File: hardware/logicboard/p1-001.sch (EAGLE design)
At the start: 25 parts, among them IC1 74LS07N, U1 TLC5940-NT, X1 HIROSE-DX10LM1-14SE

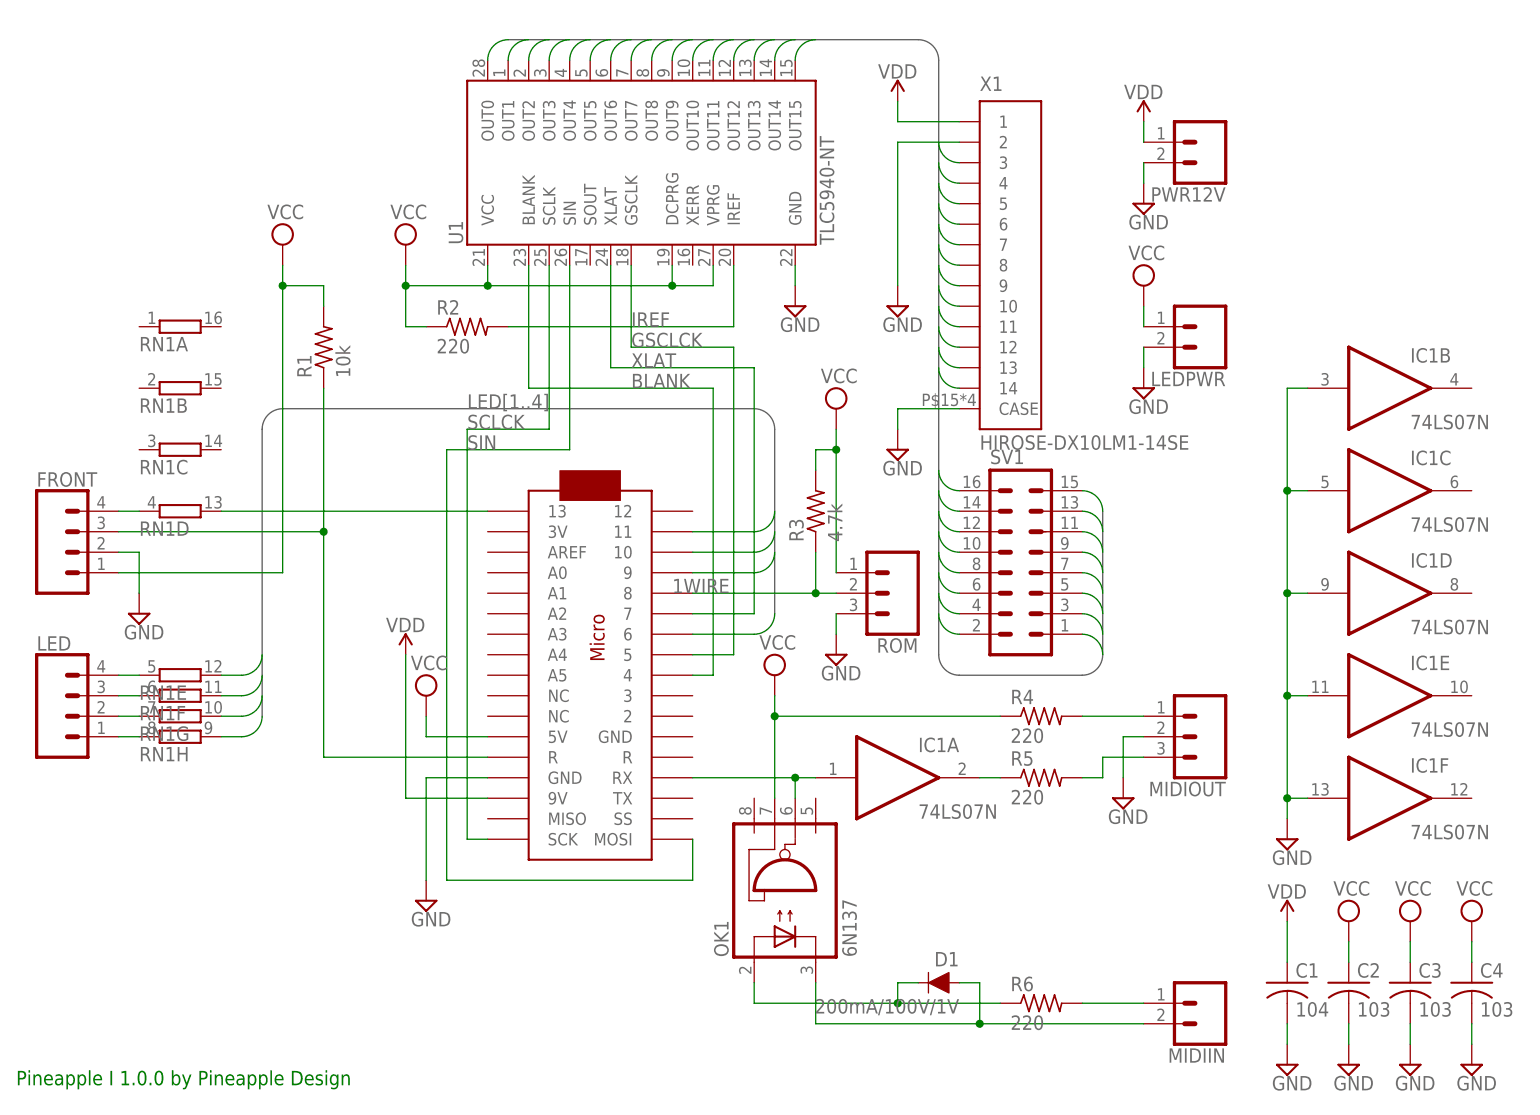
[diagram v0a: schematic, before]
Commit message: Relay.
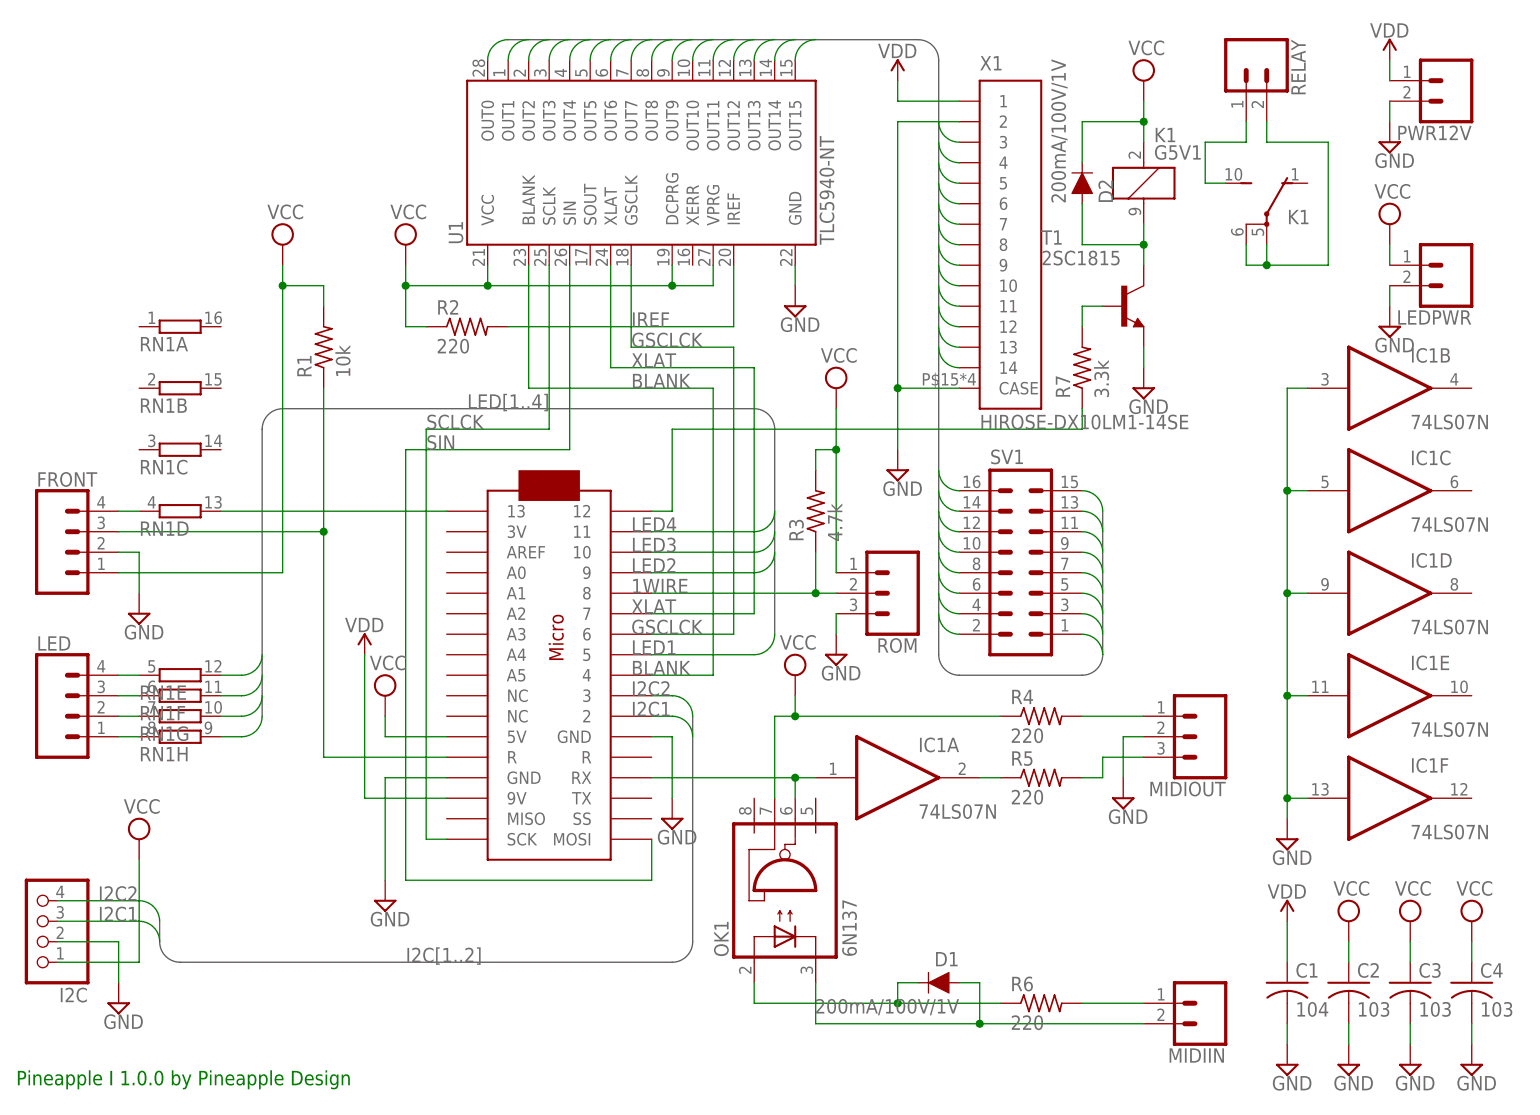
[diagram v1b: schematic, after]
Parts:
- added D2: 200mA/100V/1V, SparkFun-DiscreteSemi:DIODE-1N4148
- added I2C: (no value), pinhead:PINHD-1X4
- added K1: G5V1, relay:G5V1
- added R7: 3.3k, resistor:R-US_0204/5
- added RELAY: (no value), SparkFun-Connectors:CONN_02JST-PTH-2
- added T1: 2SC1815, transistor:2SC1815
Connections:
- new net I2C1: I2C.3, U$1.2
- new net I2C2: I2C.4, U$1.3
- new net N$14: R7.1, U$1.12
- new net N$15: R7.2, T1.B
- new net N$16: D2.A, K11.2, T1.C
- new net N$17: K12.S, RELAY.1
- new net N$18: K12.P, K12.P@1, RELAY.2
- net GND: now also I2C.2, T1.E, U$1.GND@1
- net GSCLCK: now also U$1.6; no longer U$1.5
- net LED1: now also U$1.5; no longer U$1.6
- net VCC: now also D2.C, I2C.1, K11.1
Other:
- moved on the sheet: LEDPWR, PWR12V, X1
